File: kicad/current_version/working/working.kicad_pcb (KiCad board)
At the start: 2 copper layers, 12 x 10 mm, 6 parts, among them J1 h4psmra, U1 isn280, U2 insoic14wi2cheli

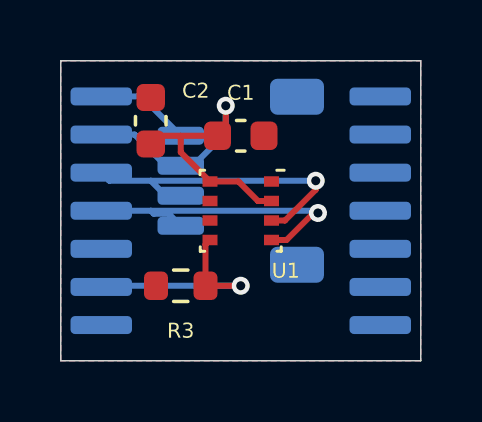
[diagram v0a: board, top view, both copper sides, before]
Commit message: ready to order boards
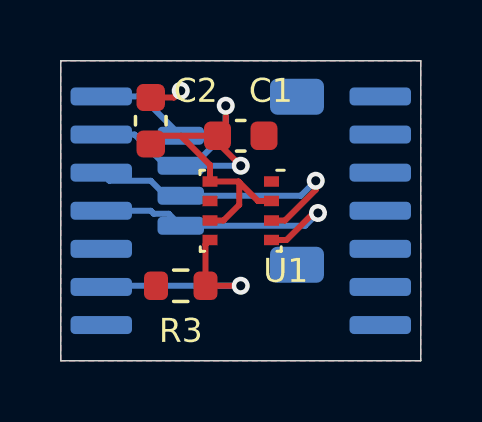
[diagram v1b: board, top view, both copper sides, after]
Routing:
- net +3V3: track 13.6 -> 18.9 mm, vias 1 -> 2
- net GND: track 3.19 -> 4.29 mm, vias 0 -> 1
- net /scl_3v3: track 10.2 -> 9.34 mm
- net /sda_3v3: track 10.6 -> 9.77 mm
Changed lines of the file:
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@@
       (outputformat 1)
       (mirror false)
-      (drillshape 1)
+      (drillshape 0)
       (scaleselection 1)
-      (outputdirectory "")
+      (outputdirectory "outputs")
     )
   )
@@
     (attr smd)
     (fp_text reference "C2" (at 1 1.5 180) (layer "F.SilkS")
-        (effects (font (size 0.5 0.5) (thickness 0.125)))
+        (effects (font (size 0.8 0.8) (thickness 0.125)))
     )
     (fp_text value "c6nf100" (at 1.5 13 180) (layer "F.Fab")
@@
     (attr smd)
     (fp_text reference "R3" (at 0 -1.5) (layer "F.SilkS")
-        (effects (font (size 0.5 0.5) (thickness 0.125)))
+        (effects (font (size 0.8 0.8) (thickness 0.125)))
     )
     (fp_text value "r6o472" (at -11.5 4) (layer "F.Fab")
@@
     (property "ki_keywords" "Bosch pressure humidity temperature environment environmental measurement digital")
     (attr smd)
-    (fp_text reference "U1" (at 2 -1.5 -180) (layer "F.SilkS")
-        (effects (font (size 0.5 0.5) (thickness 0.125)))
+    (fp_text reference "U1" (at 2 -1.5 180) (layer "F.SilkS")
+        (effects (font (size 0.8 0.8) (thickness 0.125)))
     )
     (fp_text value "isn280" (at 0.015 -9.5 -180) (layer "F.Fab")
@@
     (property "ki_keywords" "cap capacitor")
     (attr smd)
-    (fp_text reference "C1" (at 0 -1.43) (layer "F.SilkS")
-        (effects (font (size 0.5 0.5) (thickness 0.125)))
+    (fp_text reference "C1" (at 1 -1.5) (layer "F.SilkS")
+        (effects (font (size 0.8 0.8) (thickness 0.125)))
     )
     (fp_text value "c6nf100" (at 10 -0.5) (layer "F.Fab")
@@
     (property "ki_keywords" "connector")
     (attr smd)
-    (fp_text reference "J1" (at 0 3.98 90) (layer "B.SilkS")
-        (effects (font (size 1 1) (thickness 0.15)) (justify mirror))
+    (fp_text reference "J1" (at -1.5 -2 90) (layer "B.SilkS")
+        (effects (font (size 0.8 0.8) (thickness 0.15)) (justify mirror))
     )
     (fp_text value "h4psmra" (at 0 -3.98 90) (layer "B.Fab")
@@
     (pad "4" smd roundrect (at 1.5 2 270) (size 0.6 1.55) (layers "B.Cu" "B.Paste" "B.Mask") (roundrect_rratio 0.25)
       (net 4 "/scl_3v3") (pinfunction "Pin_4") (pintype "passive"))
-    (pad "MP" smd roundrect (at -2.8 -1.875 270) (size 1.2 1.8) (layers "B.Cu" "B.Paste" "B.Mask") (roundrect_rratio 0.208333))
-    (pad "MP" smd roundrect (at 2.8 -1.875 270) (size 1.2 1.8) (layers "B.Cu" "B.Paste" "B.Mask") (roundrect_rratio 0.208333))
+    (pad "MP" smd roundrect (at -2.8 -1.875 270) (size 1.2 1.8) (layers "B.Cu" "B.Paste" "B.Mask") (roundrect_rratio 0.2083333333))
+    (pad "MP" smd roundrect (at 2.8 -1.875 270) (size 1.2 1.8) (layers "B.Cu" "B.Paste" "B.Mask") (roundrect_rratio 0.2083333333))
     (model "${KICAD6_3DMODEL_DIR}/Connector_JST.3dshapes/JST_SH_SM04B-SRSS-TB_1x04-1MP_P1.00mm_Horizontal.wrl"
       (offset (xyz 0 0 0))
@@
     (fp_line (start 3.86 4.61) (end 3.86 4.37)
       (stroke (width 0.12) (type solid)) (layer "B.SilkS"))
-    (fp_line (start -5.93 -4.75) (end 5.93 -4.75)
-      (stroke (width 0.05) (type solid)) (layer "B.CrtYd"))
-    (fp_line (start -5.93 4.75) (end -5.93 -4.75)
-      (stroke (width 0.05) (type solid)) (layer "B.CrtYd"))
-    (fp_line (start 5.93 -4.75) (end 5.93 4.75)
-      (stroke (width 0.05) (type solid)) (layer "B.CrtYd"))
-    (fp_line (start 5.93 4.75) (end -5.93 4.75)
-      (stroke (width 0.05) (type solid)) (layer "B.CrtYd"))
     (fp_line (start -3.75 -4.5) (end -3.75 3.5)
       (stroke (width 0.1) (type solid)) (layer "B.Fab"))
@@
   (gr_line (start 6 -5) (end -6 -5)
     (stroke (width 0.05) (type default)) (layer "Edge.Cuts"))
+  (segment (start -3 -3.775) (end -2.225 -3.775) (width 0.2) (layer "F.Cu") (net 1))
+  (segment (start -2.225 -3.775) (end -2 -4) (width 0.2) (layer "F.Cu") (net 1))
+  (via (at -2 -4) (size 0.6) (drill 0.3) (layers "F.Cu" "B.Cu") (net 1))
   (segment (start -2 -2.5) (end -3.31 -3.81) (width 0.2) (layer "B.Cu") (net 1))
   (segment (start -3.31 -3.81) (end -4.65 -3.81) (width 0.2) (layer "B.Cu") (net 1))
+  (segment (start -0.775 -2.275) (end 0 -1.5) (width 0.2) (layer "F.Cu") (net 2))
   (segment (start -0.5 -3.5) (end -0.5 -2.775) (width 0.2) (layer "F.Cu") (net 2))
+  (segment (start -1.025 -1.525) (end -2 -2.5) (width 0.2) (layer "F.Cu") (net 2))
   (segment (start 0.575 -0.325) (end 1.025 -0.325) (width 0.2) (layer "F.Cu") (net 2))
   (segment (start -2.725 -2.5) (end -3 -2.225) (width 0.2) (layer "F.Cu") (net 2))
   (segment (start -0.5 -2.775) (end -0.775 -2.5) (width 0.2) (layer "F.Cu") (net 2))
-  (segment (start -2 -2.5) (end -2 -1.95) (width 0.2) (layer "F.Cu") (net 2))
   (segment (start -1.025 -0.975) (end -0.075 -0.975) (width 0.2) (layer "F.Cu") (net 2))
-  (segment (start -2 -1.95) (end -1.025 -0.975) (width 0.2) (layer "F.Cu") (net 2))
-  (segment (start -0.075 -0.975) (end 0.575 -0.325) (width 0.2) (layer "F.Cu") (net 2))
+  (segment (start -0.05 -0.95) (end 0.575 -0.325) (width 0.2) (layer "F.Cu") (net 2))
+  (segment (start -1.025 0.325) (end -0.575 0.325) (width 0.2) (layer "F.Cu") (net 2))
+  (segment (start -1.025 -0.975) (end -1.025 -1.525) (width 0.2) (layer "F.Cu") (net 2))
+  (segment (start -0.075 -0.975) (end -0.05 -0.95) (width 0.2) (layer "F.Cu") (net 2))
+  (segment (start -0.775 -2.5) (end -0.775 -2.275) (width 0.2) (layer "F.Cu") (net 2))
   (segment (start -2 -2.5) (end -2.725 -2.5) (width 0.2) (layer "F.Cu") (net 2))
+  (segment (start -0.05 -0.2) (end -0.05 -0.95) (width 0.2) (layer "F.Cu") (net 2))
+  (segment (start -0.575 0.325) (end -0.05 -0.2) (width 0.2) (layer "F.Cu") (net 2))
   (segment (start -2 -2.5) (end -0.775 -2.5) (width 0.2) (layer "F.Cu") (net 2))
+  (via (at 0 -1.5) (size 0.6) (drill 0.3) (layers "F.Cu" "B.Cu") (net 2))
   (via (at -0.5 -3.5) (size 0.6) (drill 0.3) (layers "F.Cu" "B.Cu") (net 2))
   (segment (start -2.5 -1.5) (end -3.54 -2.54) (width 0.2) (layer "B.Cu") (net 2))
   (segment (start -3.54 -2.54) (end -4.65 -2.54) (width 0.2) (layer "B.Cu") (net 2))
+  (segment (start 0 -1.5) (end -2 -1.5) (width 0.2) (layer "B.Cu") (net 2))
   (segment (start -2 -1.5) (end -2.5 -1.5) (width 0.2) (layer "B.Cu") (net 2))
   (segment (start -2 -1.5) (end -1.588604 -1.5) (width 0.2) (layer "B.Cu") (net 2))
@@
   (segment (start 2.5 -0.7) (end 2.5 -1) (width 0.2) (layer "F.Cu") (net 3))
   (via (at 2.5 -1) (size 0.6) (drill 0.3) (layers "F.Cu" "B.Cu") (net 3))
-  (segment (start 2.5 -1) (end -3 -1) (width 0.2) (layer "B.Cu") (net 3))
   (segment (start -2.5 -0.5) (end -3 -1) (width 0.2) (layer "B.Cu") (net 3))
+  (segment (start 2 -0.5) (end 2.5 -1) (width 0.2) (layer "B.Cu") (net 3))
   (segment (start -4.38 -1) (end -4.4 -1.02) (width 0.2) (layer "B.Cu") (net 3))
   (segment (start -3 -1) (end -4.38 -1) (width 0.2) (layer "B.Cu") (net 3))
   (segment (start -2 -0.5) (end -2.5 -0.5) (width 0.2) (layer "B.Cu") (net 3))
   (segment (start -4.4 -1.02) (end -4.4 -1.27) (width 0.2) (layer "B.Cu") (net 3))
+  (segment (start -2 -0.5) (end 2 -0.5) (width 0.2) (layer "B.Cu") (net 3))
+  (segment (start 1.525 0.975) (end 2.5 0) (width 0.2) (layer "F.Cu") (net 4))
   (segment (start 2.5 0) (end 2.573911 0.073911) (width 0.2) (layer "F.Cu") (net 4))
-  (segment (start 1.525 0.975) (end 2.5 0) (width 0.2) (layer "F.Cu") (net 4))
   (segment (start 1.025 0.975) (end 1.525 0.975) (width 0.2) (layer "F.Cu") (net 4))
   (via (at 2.573911 0.073911) (size 0.6) (drill 0.3) (layers "F.Cu" "B.Cu") (net 4))
@@
   (segment (start -2.9 0.1) (end -3 0) (width 0.2) (layer "B.Cu") (net 4))
   (segment (start -2.4 0.1) (end -2.9 0.1) (width 0.2) (layer "B.Cu") (net 4))
+  (segment (start 2.147822 0.5) (end -2 0.5) (width 0.2) (layer "B.Cu") (net 4))
   (segment (start -2 0.5) (end -2.4 0.1) (width 0.2) (layer "B.Cu") (net 4))
-  (segment (start 2.573911 0.073911) (end 2.5 0) (width 0.2) (layer "B.Cu") (net 4))
-  (segment (start 2.5 0) (end -3 0) (width 0.2) (layer "B.Cu") (net 4))
+  (segment (start 2.573911 0.073911) (end 2.147822 0.5) (width 0.2) (layer "B.Cu") (net 4))
   (segment (start -1.175 1.125) (end -1.025 0.975) (width 0.2) (layer "F.Cu") (net 6))
   (segment (start -1.175 2.5) (end -1.175 1.125) (width 0.2) (layer "F.Cu") (net 6))
@@
   (segment (start 0 2.5) (end -4.61 2.5) (width 0.2) (layer "B.Cu") (net 6))
   (zone (net 1) (net_name "GND") (layers "F&B.Cu") (hatch edge 0.5)
-    (connect_pads (clearance 0.5))
-    (min_thickness 0.25) (filled_areas_thickness no)
-    (fill yes (thermal_gap 0.5) (thermal_bridge_width 0.5))
+    (connect_pads (clearance 0.25))
+    (min_thickness 0.2) (filled_areas_thickness no)
+    (fill yes (thermal_gap 0.25) (thermal_bridge_width 0.25))
     (polygon
       (pts
